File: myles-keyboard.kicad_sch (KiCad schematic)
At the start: 52 parts, among them J1 TRRS, J2 OLED, SW00 Key, SW01 Key, SW02 Key, SW03 Key, SW04 Key, SW05 Key, SW10 Key, SW11 Key, SW12 Key, SW13 Key, SW14 Key, SW15 Key, SW16 Key, SW17 Key, SW18 Key, SW20 Key, SW21 Key, SW22 Key, SW23 Key, SW24 Key, SW25 Key, SW26 Key, SW27 Key, SW28 Key, SW30 Key, SW31 Key, SW32 Key, SW33 Key, SW34 Key, SW35 Key, SW36 Key, SW37 Key, SW38 Key, SW40 Key, SW41 Key, SW42 Key, SW43 Key, SW44 Key, SW45 Key, SW46 Key, SW47 Key, SW48 Key, U1 ProMicro

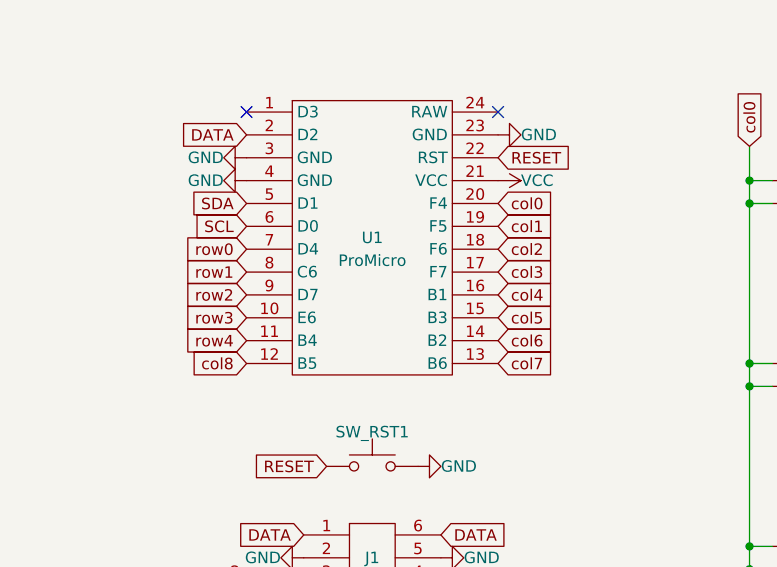
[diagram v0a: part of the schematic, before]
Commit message: draft wiring
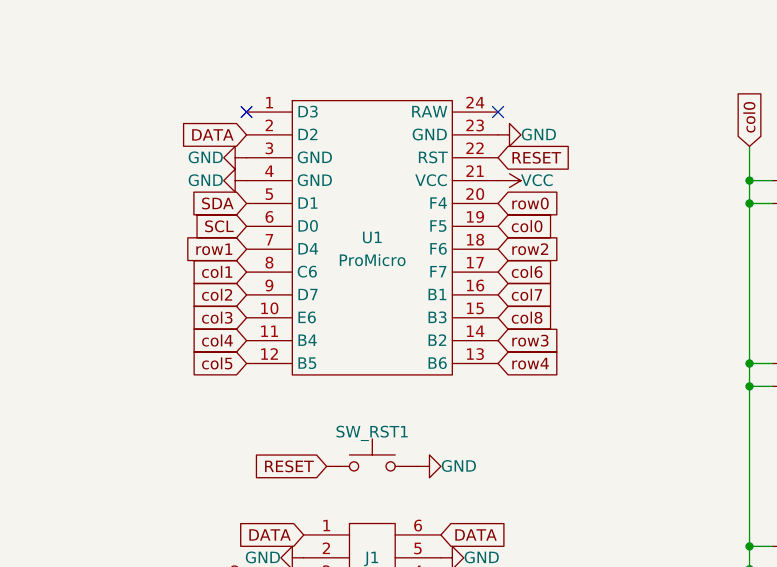
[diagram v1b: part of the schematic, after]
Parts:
- SW10, SW20: footprint myles-keyboard:Key -> myles-keyboard:KeyLeft
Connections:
- net col0: now also U1.19 (F5); no longer U1.20 (F4)
- net col1: now also U1.8 (C6); no longer U1.19 (F5)
- net col2: now also U1.9 (D7); no longer U1.18 (F6)
- net col3: now also U1.10 (E6); no longer U1.17 (F7)
- net col4: now also U1.11 (B4); no longer U1.16 (B1)
- net col5: now also U1.12 (B5); no longer U1.15 (B3)
- net col6: now also U1.17 (F7); no longer U1.14 (B2)
- net col7: now also U1.16 (B1); no longer U1.13 (B6)
- net col8: now also U1.15 (B3); no longer U1.12 (B5)
- net row0: now also U1.20 (F4); no longer U1.7 (D4)
- net row1: now also U1.7 (D4); no longer U1.8 (C6)
- net row2: now also U1.18 (F6); no longer U1.9 (D7)
- net row3: now also U1.14 (B2); no longer U1.10 (E6)
- net row4: now also U1.13 (B6); no longer U1.11 (B4)
